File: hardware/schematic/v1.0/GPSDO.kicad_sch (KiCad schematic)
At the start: 78 parts, among them J1 USB_C_Receptacle_USB2.0_16P, J2 Conn_Coaxial, Q1 AO3400A, SW1 SW_Push, SW2 SW_Push, U1 STM32G431KBUx, U2 OCXO-10M, U3 SKG123N, U4 IPEX1, U5 BQ25890, U6 TPS7A8901, U7 CH340E, U8 LMK1C1102, Y1 Crystal_GND24

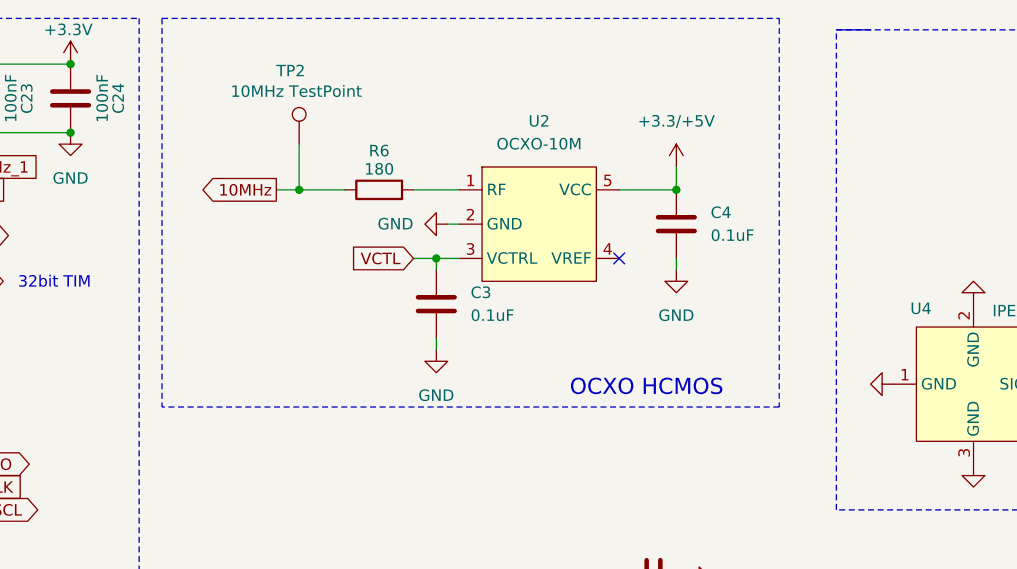
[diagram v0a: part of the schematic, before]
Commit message: sch update
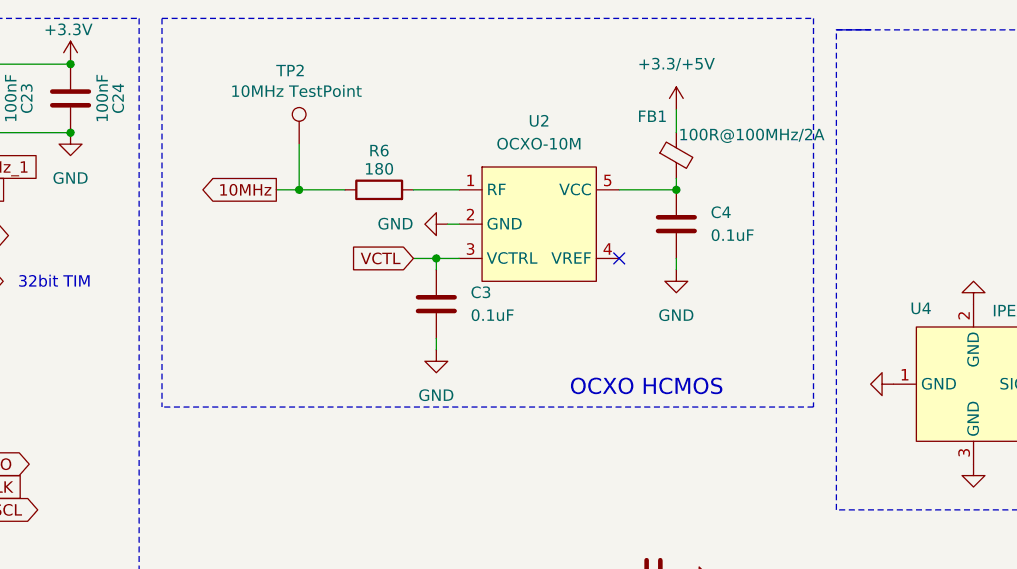
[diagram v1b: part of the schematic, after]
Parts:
- added FB1: 100R@100MHz/2A, Inductor_SMD:L_1206_3216Metric, symbol Device:FerriteBead_Small
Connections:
- net +3.3/+5V: now also FB1.1; no longer C4.1, U2.5 (VCC)
- new net: C4.1, FB1.2, U2.5 (VCC)
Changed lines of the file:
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@@
 	(polyline
 		(pts
-			(xy 157.48 13.97) (xy 157.48 57.15)
+			(xy 161.29 13.97) (xy 161.29 57.15)
 		)
 		(stroke
@@
 	(wire
 		(pts
+			(xy 146.05 31.75) (xy 146.05 33.02)
+		)
+		(stroke
+			(width 0)
+			(type default)
+		)
+	)
+	(wire
+		(pts
 			(xy 71.12 170.18) (xy 71.12 173.99)
 		)
@@
 	(polyline
 		(pts
-			(xy 157.48 57.15) (xy 88.9 57.15)
+			(xy 161.29 57.15) (xy 88.9 57.15)
 		)
 		(stroke
@@
 	(wire
 		(pts
-			(xy 146.05 30.48) (xy 146.05 33.02)
+			(xy 146.05 24.13) (xy 146.05 26.67)
 		)
 		(stroke
@@
 	(polyline
 		(pts
-			(xy 88.9 13.97) (xy 157.48 13.97)
+			(xy 88.9 13.97) (xy 161.29 13.97)
 		)
 		(stroke
@@
 	(symbol
 		(lib_id "power:+3.3V")
-		(at 146.05 30.48 0)
+		(at 146.05 24.13 0)
 		(unit 1)
 		(body_style 1)
@@
 		(fields_autoplaced yes)
 		(property "Reference" "#PWR028"
-			(at 146.05 34.29 0)
+			(at 146.05 27.94 0)
 			(hide yes)
 			(show_name no)
@@
 		)
 		(property "Value" "+3.3/+5V"
-			(at 146.05 25.4 0)
+			(at 146.05 19.05 0)
 			(show_name no)
 			(do_not_autoplace no)
@@
 		)
 		(property "Footprint" ""
-			(at 146.05 30.48 0)
+			(at 146.05 24.13 0)
 			(hide yes)
 			(show_name no)
@@
 		)
 		(property "Datasheet" ""
-			(at 146.05 30.48 0)
+			(at 146.05 24.13 0)
 			(hide yes)
 			(show_name no)
@@
 		)
 		(property "Description" "Power symbol creates a global label with name \"+3.3V\""
-			(at 146.05 30.48 0)
+			(at 146.05 24.13 0)
 			(hide yes)
 			(show_name no)
@@
 					(unit 1)
 				)
+			)
+		)
+	)
+	(symbol
+		(lib_id "Device:FerriteBead_Small")
+		(at 146.05 29.21 0)
+		(unit 1)
+		(body_style 1)
+		(exclude_from_sim no)
+		(in_bom yes)
+		(on_board yes)
+		(in_pos_files yes)
+		(dnp no)
+		(property "Reference" "FB1"
+			(at 141.732 24.892 0)
+			(show_name no)
+			(do_not_autoplace no)
+			(effects
+				(font
+					(size 1.27 1.27)
+				)
+				(justify left)
+			)
+		)
+		(property "Value" "100R@100MHz/2A"
+			(at 146.304 26.924 0)
+			(show_name no)
+			(do_not_autoplace no)
+			(effects
+				(font
+					(size 1.27 1.27)
+				)
+				(justify left)
+			)
+		)
+		(property "Footprint" "Inductor_SMD:L_1206_3216Metric"
+			(at 144.272 29.21 90)
+			(hide yes)
+			(show_name no)
+			(do_not_autoplace no)
+			(effects
+				(font
+					(size 1.27 1.27)
+				)
+			)
+		)
+		(property "Datasheet" ""
+			(at 146.05 29.21 0)
+			(hide yes)
+			(show_name no)
+			(do_not_autoplace no)
+			(effects
+				(font
+					(size 1.27 1.27)
+				)
+			)
+		)
+		(property "Description" "OCXO VCC 滤波磁珠，DCR 不大于 0.02 欧，额定电流不小于 2 A"
+			(at 146.05 29.21 0)
+			(hide yes)
+			(show_name no)
+			(do_not_autoplace no)
+			(effects
+				(font
+					(size 1.27 1.27)
+				)
+			)
+		)
+		(pin "1"
+		)
+		(pin "2"
+		)
+		(instances
+			(project "GPSDO"
+				(path "/bb9f04d0-06e2-4b9f-871a-754dc45b8574"
+					(reference "FB1")
+					(unit 1)
+				)
